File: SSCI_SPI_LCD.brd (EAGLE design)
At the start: 42 x 35 mm, 28 parts, among them IC3 74LVC541_RGY, X1 TSW-108-02-S-S, X2 TSW-108-02-S-S

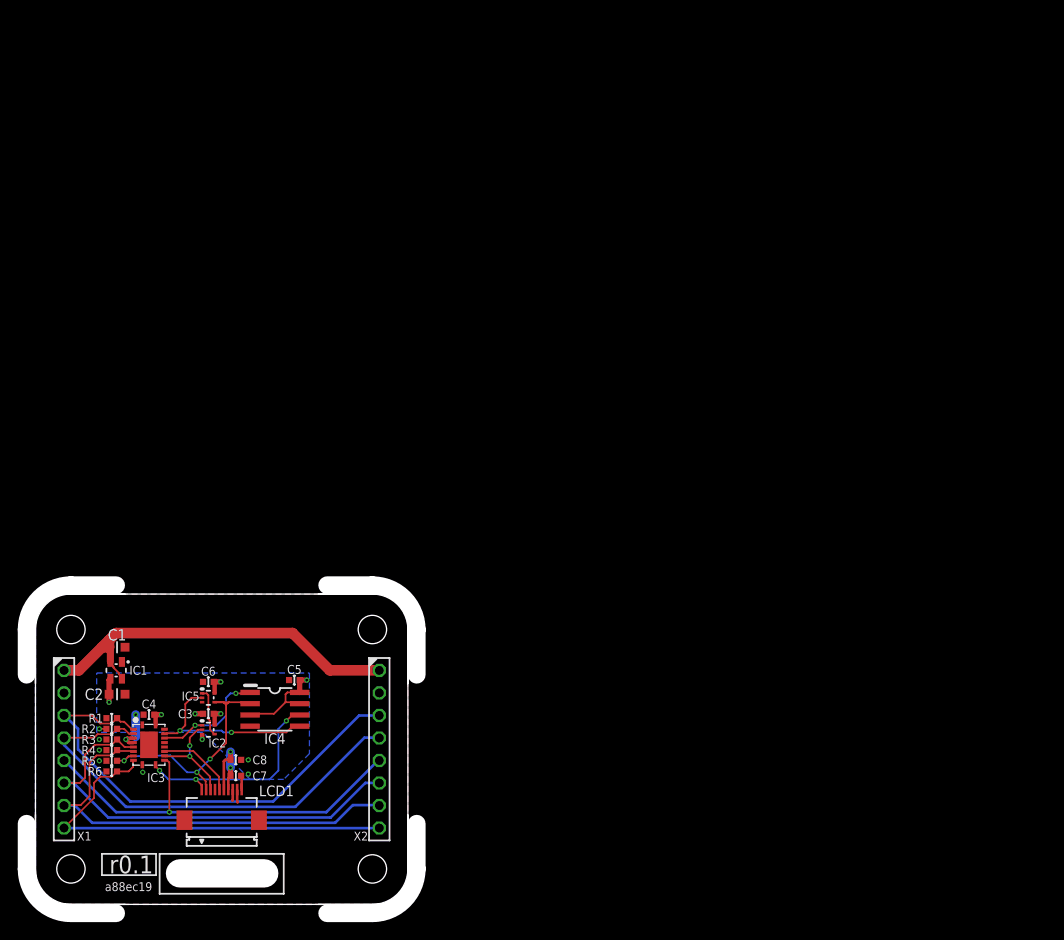
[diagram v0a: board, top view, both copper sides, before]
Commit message: revision 0.1
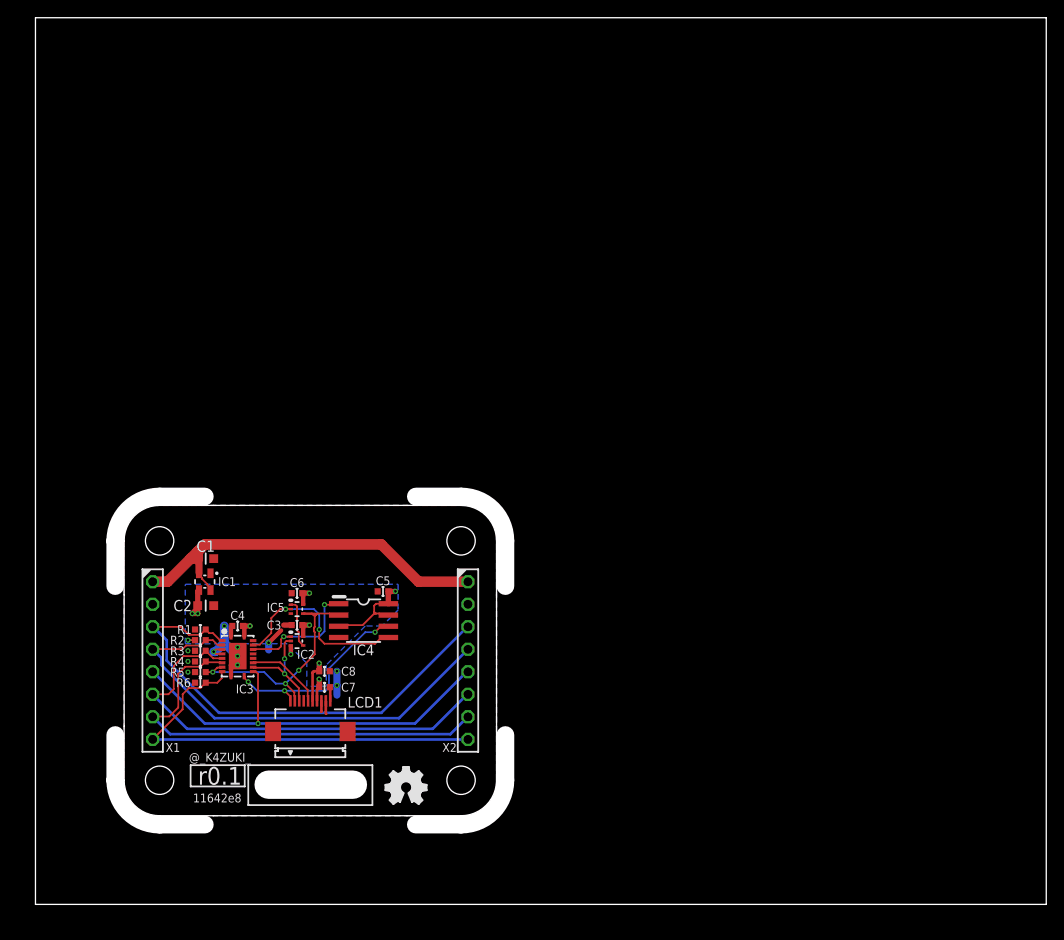
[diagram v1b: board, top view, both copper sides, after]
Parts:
- added ICON2: (no value), mylib:ICON_OSHW
- GIT1: value a88ec19 -> 11642e8
- moved C2 14.1 mm to (19.2, 33.7)
- moved C1 14.1 mm to (19.2, 39.0)
- moved C3 14.1 mm to (29.5, 31.5)
- moved C4 14.1 mm to (22.8, 31.4)
- moved C6 14.1 mm to (29.5, 35.1)
- moved C7 14.1 mm to (32.6, 24.5)
- moved C8 14.1 mm to (32.6, 26.3)
- moved GIT1 14.1 mm to (20.5, 12.0)
- moved IC1 14.1 mm to (19.1, 36.4)
- moved IC2 14.1 mm to (29.5, 29.7)
- moved IC3 14.1 mm to (22.8, 28.0)
- moved IC4 14.1 mm to (37.0, 32.0)
- moved ICON1 14.1 mm to (20.8, 14.5)
- moved LCD1 14.1 mm to (31.0, 19.5)
- moved P1 14.1 mm to (48.0, 14.0)
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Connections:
- net GND: now also LCD1.PAD1, LCD1.PAD2
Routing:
- net GND: track 10.2 -> 22.6 mm, vias 10 -> 12
- net SCK-: track 24.3 -> 22.7 mm
- net !CSR!-: track 13.8 -> 14.9 mm
- net MOSI-: track 21.2 -> 22.0 mm
- net 3.3V: track 30.1 -> 30.0 mm, vias 8 -> 9
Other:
- board size 42 x 35 mm -> 114 x 100 mm
- board text added: "@_K4ZUKI_"
